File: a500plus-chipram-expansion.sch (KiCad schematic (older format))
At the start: 10 parts, among them J1 Expansion Header, J2 Enable, U1 XRAS(0) 512KB, U2 XRAS(1) 512KB

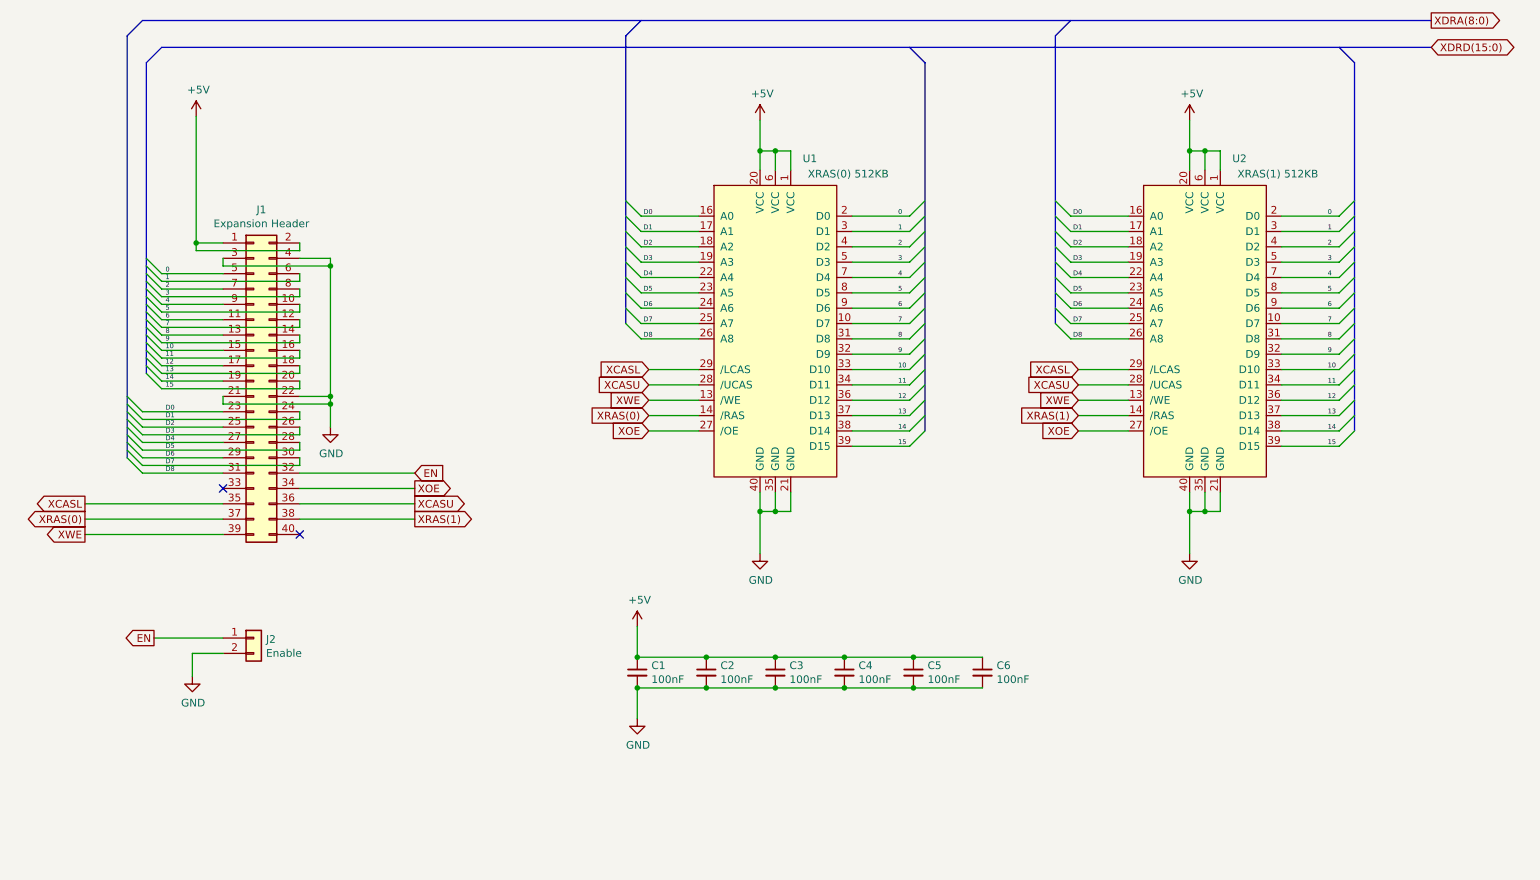
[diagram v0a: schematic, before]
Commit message: v1.1
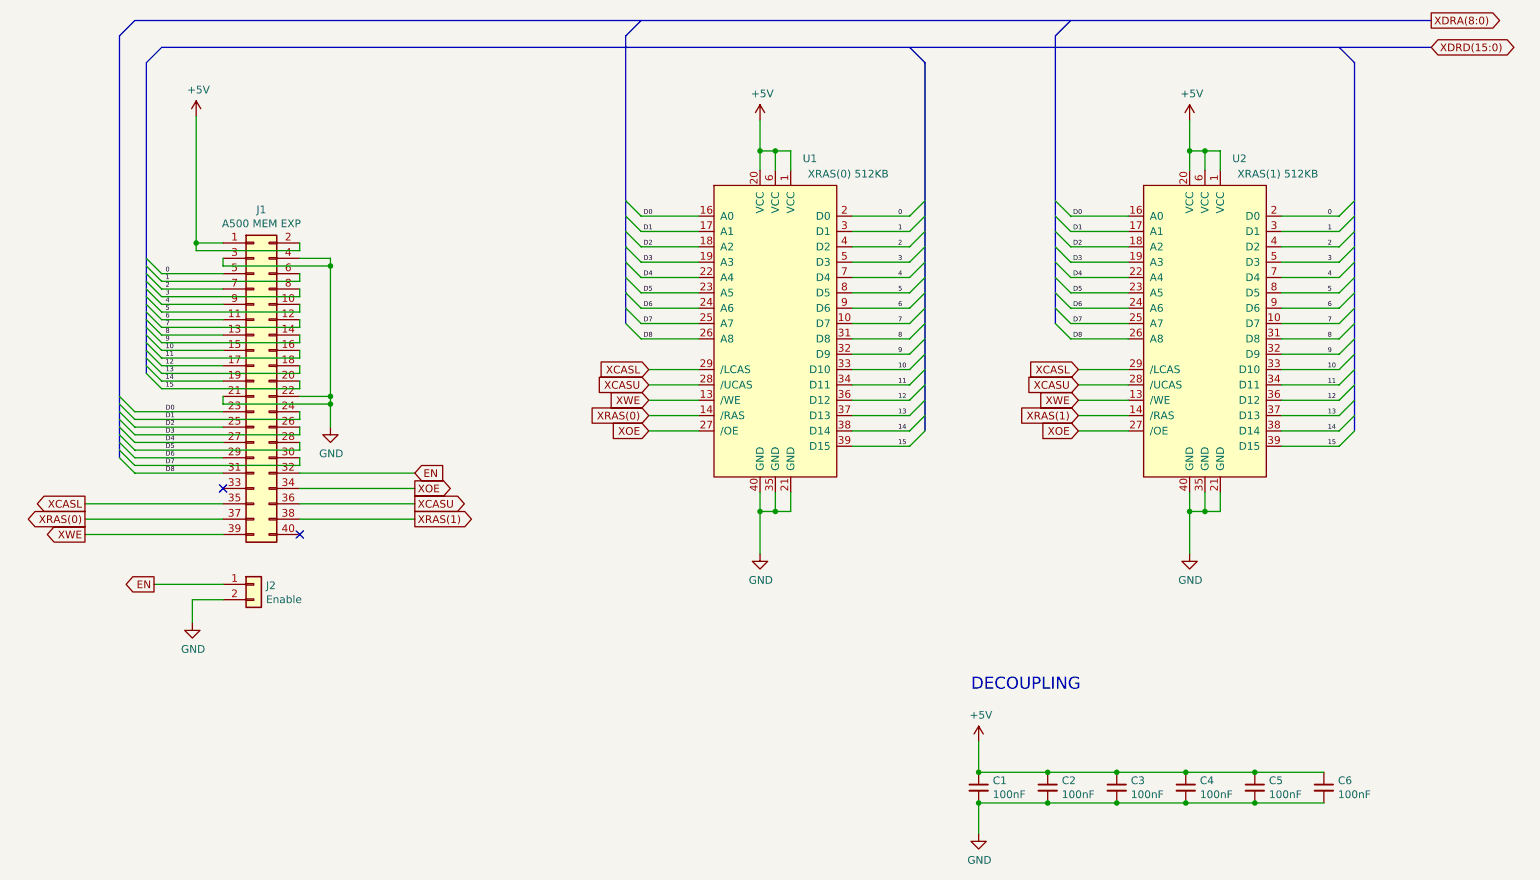
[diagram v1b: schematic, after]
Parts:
- J1: value Expansion Header -> A500 MEM EXP
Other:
- note added: "DECOUPLING"
- moved on the sheet: C1, C2, C3, C4, C5, C6, J2
